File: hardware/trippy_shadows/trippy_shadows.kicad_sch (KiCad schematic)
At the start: 32 parts, among them J1 ISP, J10 JST conn, J2 GPIO, J3 DEBUG, J4 PWR, J5 JST conn, J6 JST conn, J7 JST conn, J8 JST conn, J9 JST conn, U1 ATmega328P-AU, U2 CN5711, U3 CN5711, U4 CN5711, U5 CN5711, U6 CN5711, U7 CN5711

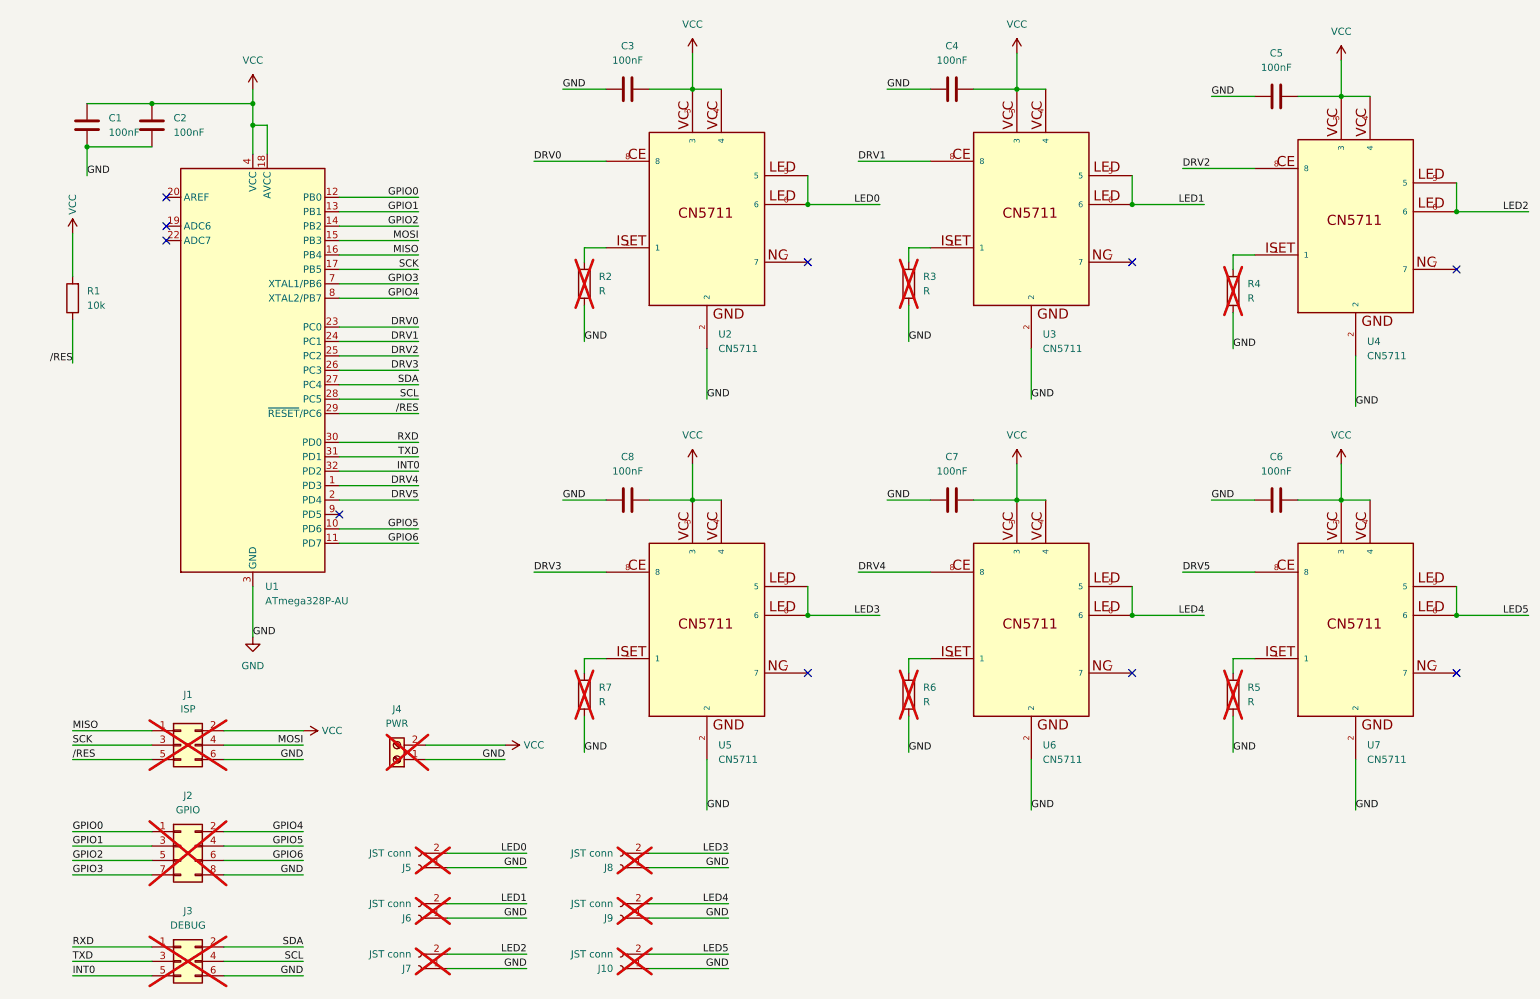
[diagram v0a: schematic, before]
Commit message: Commit latest board design
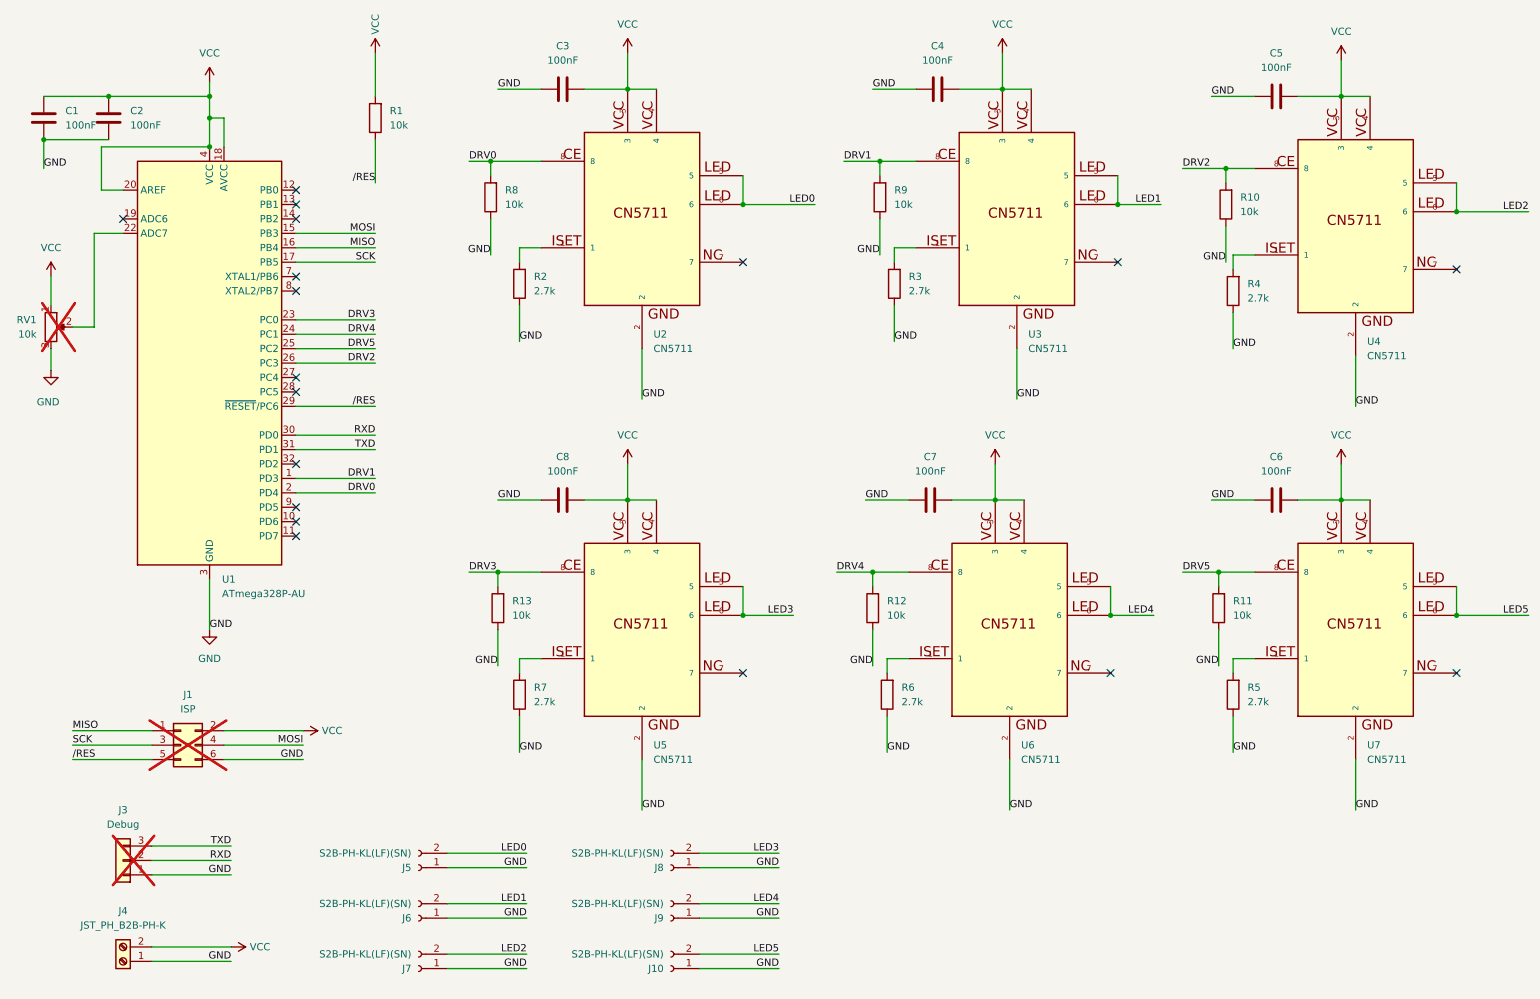
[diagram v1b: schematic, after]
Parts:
- removed J2: GPIO, Connector_PinHeader_2.54mm:PinHeader_2x04_P2.54mm_Vertical, symbol Connector_Generic:Conn_02x04_Odd_Even
- removed J3: DEBUG, Connector_PinHeader_2.54mm:PinHeader_2x03_P2.54mm_Vertical, symbol Connector_Generic:Conn_02x03_Odd_Even
- added J3: Debug, Connector_PinHeader_2.54mm:PinHeader_1x03_P2.54mm_Vertical, symbol Connector_Generic:Conn_01x03
- added R10, R11, R12, R13, R8, R9: 10k, Resistor_SMD:R_0805_2012Metric, symbol Device:R
- added RV1: 10k, Potentiometer_THT:Potentiometer_Alps_RK09K_Single_Vertical, symbol Device:R_Potentiometer
- J10, J5, J6, J7, J8, J9: value JST conn -> S2B-PH-KL(LF)(SN); footprint Connector_JST:JST_PH_B2B-PH-K_1x02_P2.00mm_Vertical -> Connector_JST:JST_PH_S2B-PH-K_1x02_P2.00mm_Horizontal; now fitted
- J4: value PWR -> JST_PH_B2B-PH-K; footprint TerminalBlock:TerminalBlock_bornier-2_P5.08mm -> Connector_JST:JST_PH_B2B-PH-K_1x02_P2.00mm_Vertical; now fitted
- R2, R3, R4, R5, R6, R7: value R -> 2.7k; now fitted
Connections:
- net DRV0: now also U1.2 (PD4), R8.2; no longer U1.23 (PC0)
- net DRV1: now also U1.1 (PD3), R9.2; no longer U1.24 (PC1)
- net DRV2: now also U1.26 (PC3), R10.2; no longer U1.25 (PC2)
- net DRV3: now also U1.23 (PC0), R13.2; no longer U1.26 (PC3)
- net DRV4: now also U1.24 (PC1), R12.2; no longer U1.1 (PD3)
- net DRV5: now also U1.25 (PC2), R11.2; no longer U1.2 (PD4)
- net GND: now also J3.1 (Pin_1), R10.1, R11.1, R12.1, R13.1, R8.1, R9.1, RV1.3
- net RXD: now also J3.2 (Pin_2)
- net TXD: now also J3.3 (Pin_3)
- net VCC: now also U1.20 (AREF), RV1.1
- net at U1.22 (ADC7): now also RV1.2
- net GPIO0: no longer names the net of U1.12 (PB0)
- net GPIO1: no longer names the net of U1.13 (PB1)
- net GPIO2: no longer names the net of U1.14 (PB2)
- net GPIO3: no longer names the net of U1.7 (XTAL1/PB6)
- net GPIO4: no longer names the net of U1.8 (XTAL2/PB7)
- net GPIO5: no longer names the net of U1.10 (PD6)
- net GPIO6: no longer names the net of U1.11 (PD7)
- net INT0: no longer names the net of U1.32 (PD2)
- net SCL: no longer names the net of U1.28 (PC5)
- net SDA: no longer names the net of U1.27 (PC4)
- no-connect marks 10 -> 18
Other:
- moved on the sheet: C1, C2, C3, C4, C7, C8, R1, U1, U2, U3, U5, U6
